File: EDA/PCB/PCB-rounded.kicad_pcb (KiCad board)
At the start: 2 copper layers, 69.5 x 45.1 mm, 14 parts, among them J1 Conn_01x08_Female, J2 Screw_Terminal_01x02, J3 Screw_Terminal_01x03, J4 Conn_01x02_Male, J5 Conn_01x03_Male, U1 PC817, U2 PC817, U3 WeMos D1 Mini, U4 PC817

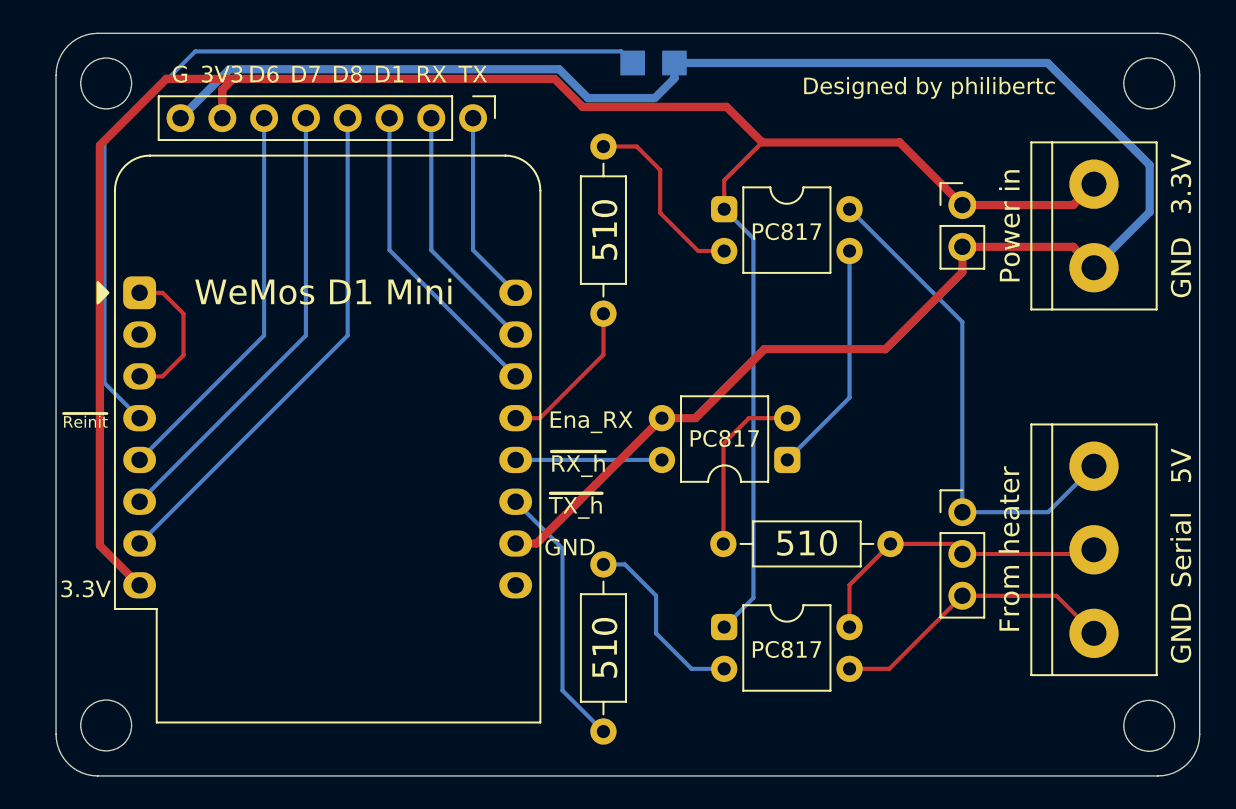
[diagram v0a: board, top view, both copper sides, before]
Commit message: v1.3 (v3 of first iteration)
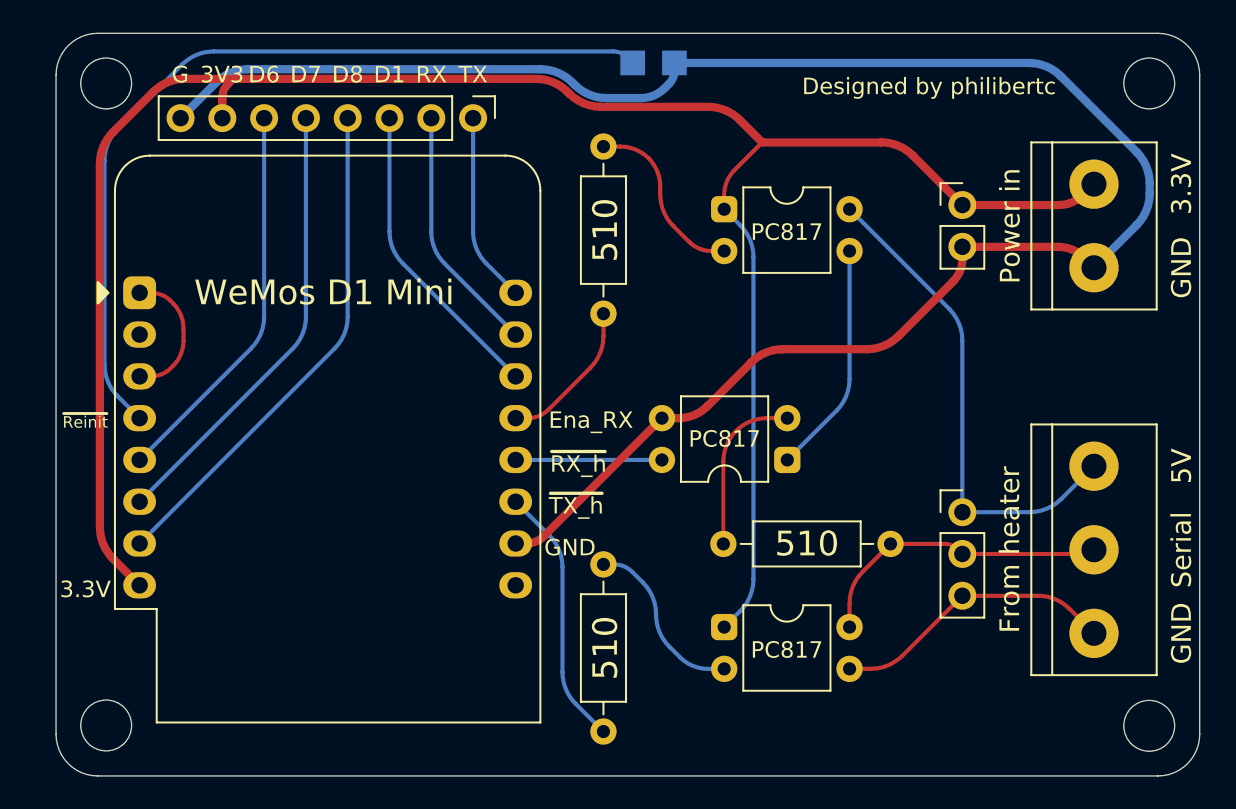
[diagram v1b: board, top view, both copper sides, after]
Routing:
- net Net-(J1-Pad8): track 116.6 -> 115.0 mm
- net Net-(J1-Pad7): track 128.2 -> 126.8 mm
- net Net-(TP1-Pad1): track 53.1 -> 52.2 mm
